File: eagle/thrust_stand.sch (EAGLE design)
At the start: 28 parts, among them IC1 7805TV, Q1 16Mhz, Q2 IRF510, T1 2N3904, U2 ATMEGA328P_PDIP

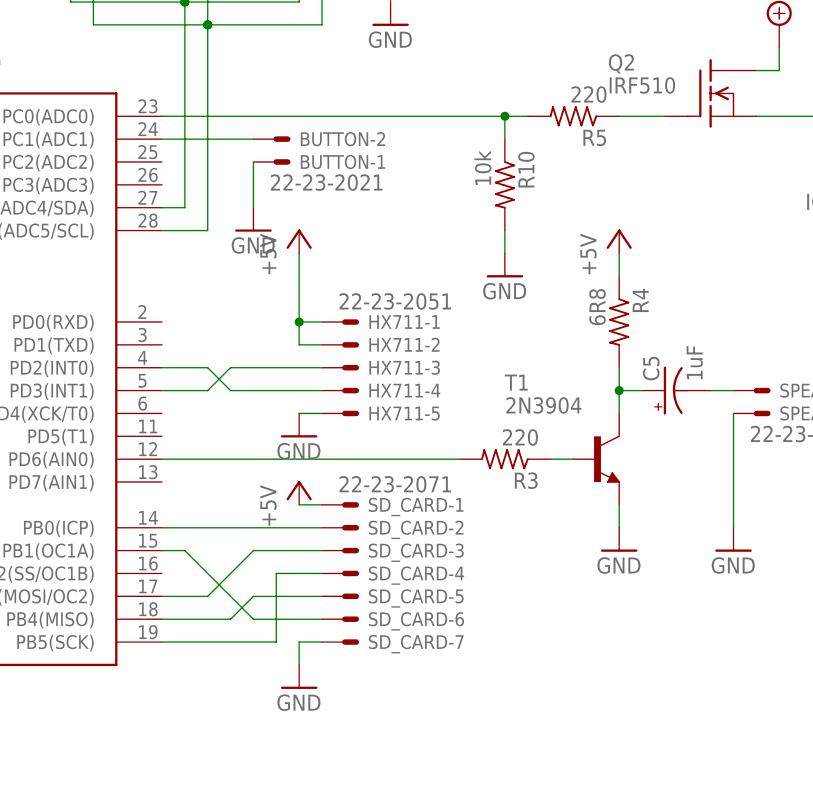
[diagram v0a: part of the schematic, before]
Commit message: rotary encoder schemo and codes
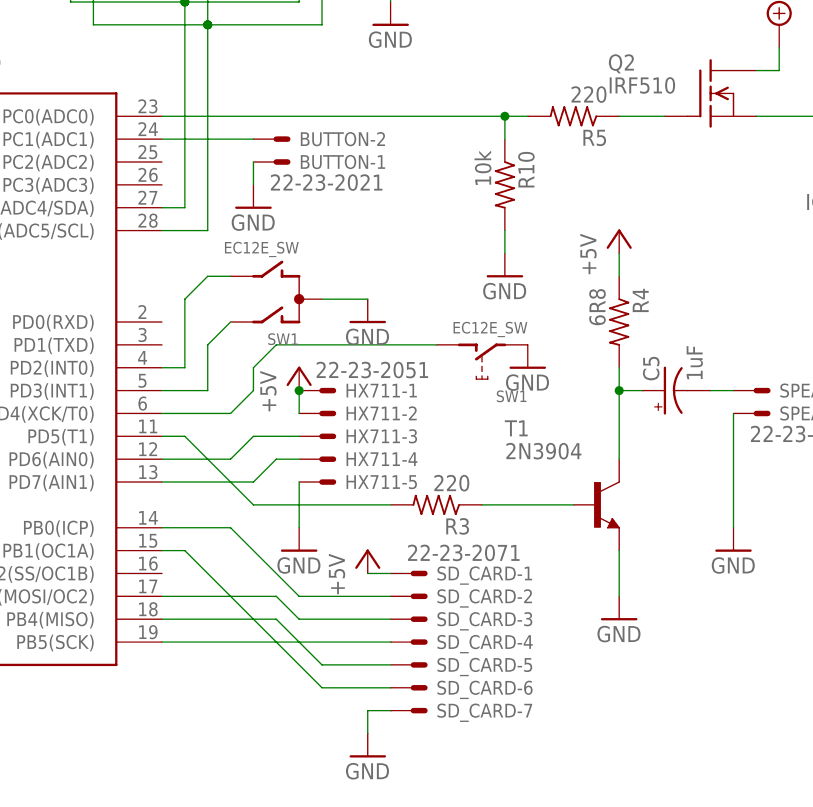
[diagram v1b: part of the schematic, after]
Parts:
- added SW1: EC12E_SW, switch-alps:EC12E_SW
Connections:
- new net N$19: SW1G$1.B, U2.PD2(INT0)
- new net N$20: SW1G$1.A, U2.PD3(INT1)
- new net N$22: SW1G$2.1, U2.PD4(XCK/T0)
- net GND: now also SW1G$1.C, SW1G$2.2
- net N$13: now also U2.PD5(T1); no longer U2.PD6(AIN0)
- net N$3: now also U2.PD6(AIN0); no longer U2.PD3(INT1)
- net N$6: now also U2.PD7(AIN1); no longer U2.PD2(INT0)
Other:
- moved on the sheet: HX711-1, HX711-2, HX711-3, HX711-4, HX711-5, R3, SD_CARD-1, SD_CARD-2, SD_CARD-3, SD_CARD-4, SD_CARD-5, SD_CARD-6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
